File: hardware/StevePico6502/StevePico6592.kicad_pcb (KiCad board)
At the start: 2 copper layers, 145.3 x 124 mm, 41 parts, among them J1 GPIOB, J10 FTDI Power, J2 GPIOA, J3 Conn_02x16_Odd_Even, J4 ROM SELECT, J5 RAM SELECT, J6 Expansion, J7 IO SELECT, J8 CLK SELECT, J9 FTDI Connector, SW1 SW_Push, U1 W65C02S, U2 28C256, U3 CY62256-70PC, U4 W65C22S, U5 74HC00, U6 W6551, X1 CXO_DIP14, Y1 1.843

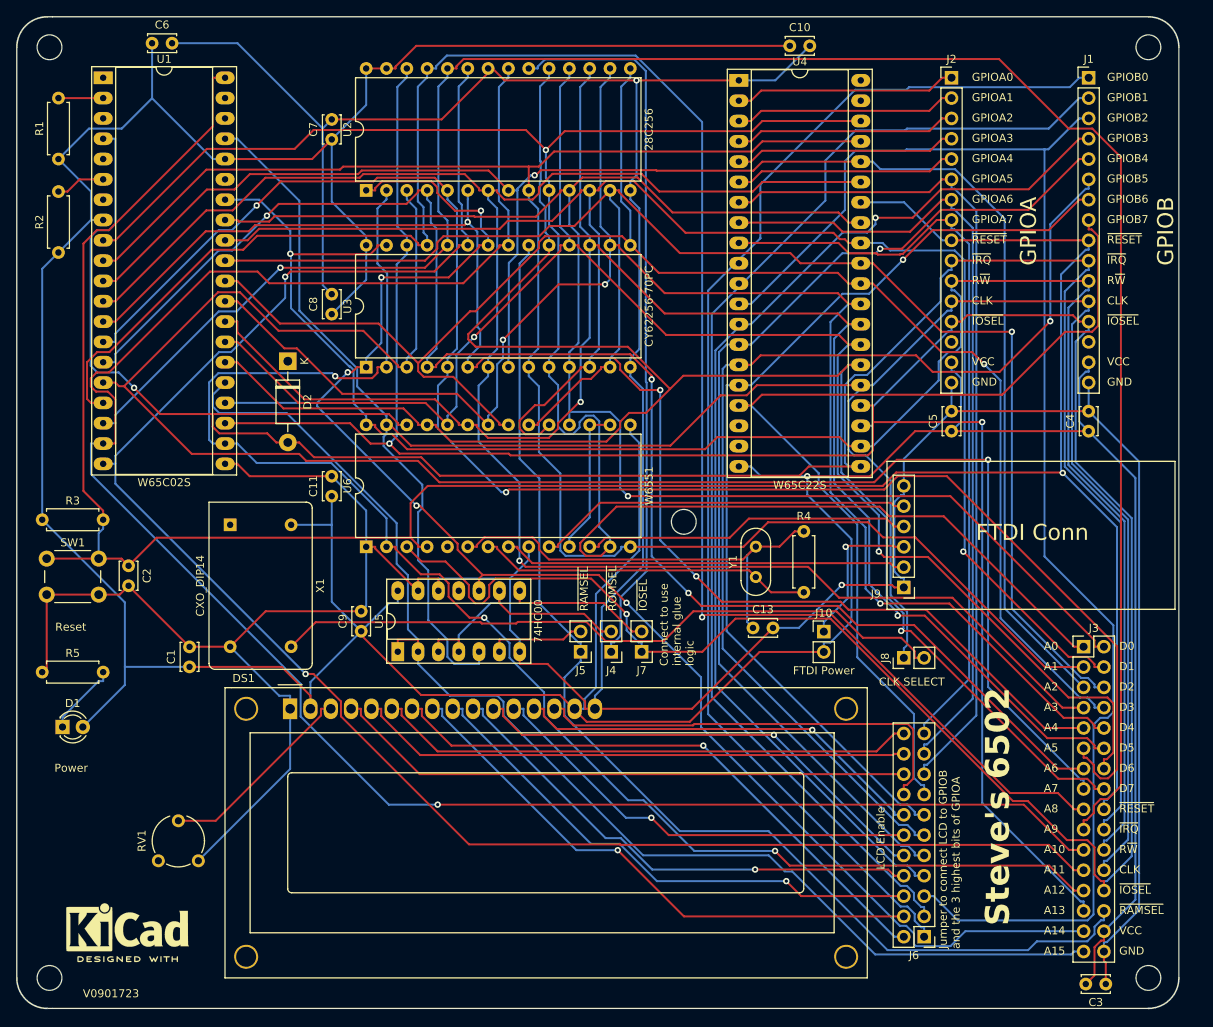
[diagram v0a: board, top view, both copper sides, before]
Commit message: 'V091723'
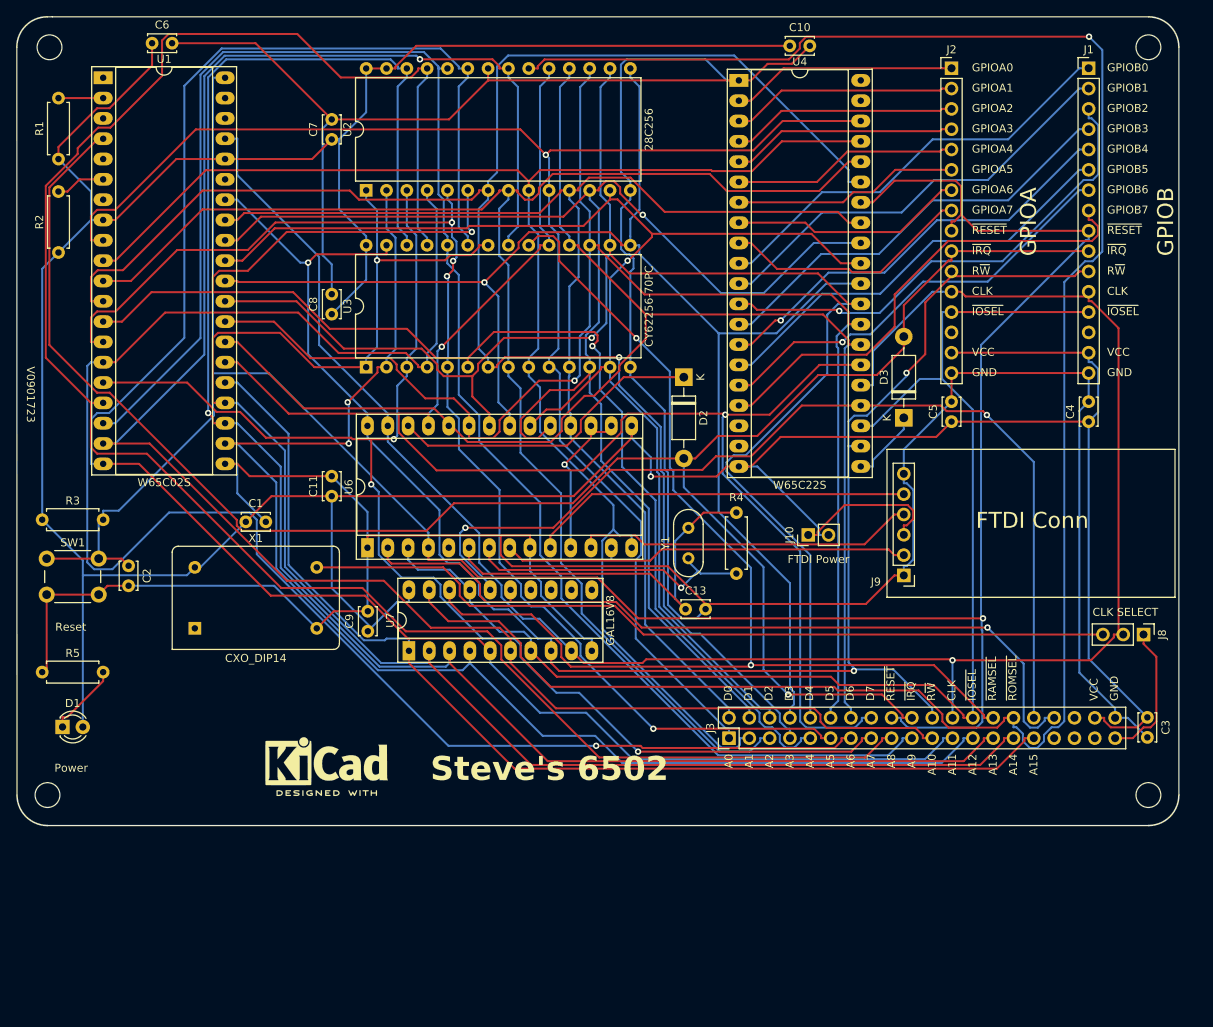
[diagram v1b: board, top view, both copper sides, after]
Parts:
- removed DS1: WC1602A, Display:WC1602A
- removed J4: ROM SELECT, Connector_PinHeader_2.54mm:PinHeader_1x02_P2.54mm_Vertical
- removed J5: RAM SELECT, Connector_PinHeader_2.54mm:PinHeader_1x02_P2.54mm_Vertical
- removed J6: Expansion, Connector_PinHeader_2.54mm:PinHeader_2x11_P2.54mm_Vertical
- removed J7: IO SELECT, Connector_PinHeader_2.54mm:PinHeader_1x02_P2.54mm_Vertical
- removed RV1: 10k, Potentiometer_THT:Potentiometer_Piher_PT-6-V_Vertical
- removed U5: 74HC00, Package_DIP:DIP-14_W7.62mm_Socket_LongPads
- added D3: SB140, Diode_THT:D_DO-41_SOD81_P10.16mm_Horizontal, F.Cu at (159.8, 83.2)
- added U7: GAL16V8, Package_DIP:DIP-20_W7.62mm_Socket_LongPads, F.Cu at (97.9, 112.3)
- J3: value Conn_02x16_Odd_Even -> Conn_02x20_Odd_Even; footprint Connector_PinHeader_2.54mm:PinHeader_2x16_P2.54mm_Vertical -> Connector_PinHeader_2.54mm:PinHeader_2x20_P2.54mm_Vertical
- J8: footprint Connector_PinHeader_2.54mm:PinHeader_1x02_P2.54mm_Vertical -> Connector_PinHeader_2.54mm:PinHeader_1x03_P2.54mm_Vertical
- U6: footprint Package_DIP:DIP-28_W15.24mm -> Package_DIP:DIP-28_W15.24mm_Socket_LongPads
- moved D2 49.5 mm to (132.3, 78.1)
- moved J3 45.8 mm to (137.9, 123.2), turned to 90 degrees
- moved C3 34.2 mm to (190.2, 120.6), turned to -90 degrees
- moved REF** 32.4 mm to (87.6, 126.1)
- moved J8 30.1 mm to (189.7, 110.2), turned to -90 degrees
- moved C1 19.4 mm to (77.5, 96.2), turned to 0 degrees
- moved X1 13.7 mm to (71.2, 109.5), turned to 0 degrees
- moved J10 12.2 mm to (147.8, 97.8), turned to 90 degrees
- moved C13 8.75 mm to (132.5, 107.1)
- moved R4 8.75 mm to (138.8, 102.6)
- moved Y1 8.75 mm to (132.8, 100.7)
- moved J9 1.50 mm to (159.8, 102.8)
- moved C4 1.19 mm to (182.9, 83.6)
- moved C5 1.19 mm to (165.7, 83.6)
- moved J1 1.19 mm to (182.9, 39.5)
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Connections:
- J3 pad 30: VCC -> /~{ROMSEL}
- J3 pad 32: GND -> /6522SEL
- J8 pad 1: /CLK -> /CLK_ALT
- J8 pad 2: /CLK_INT -> /CLK
- U4 pad 21: /~{IRQ} -> Net-(D3-K)
- U4 pad 24: /A13 -> /6522SEL
- U6 pad 2: /A12 -> /ACIASEL
- U6 pad 26: /~{IRQ} -> Net-(D2-K)
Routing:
- net /~{ROMSEL}: track 90.5 -> 255.3 mm, vias 0 -> 1
- net /6522SEL: track 0.00 -> 121.9 mm, vias 0 -> 2
- net /GPIOB2: track 180.4 -> 61.5 mm, vias 0 -> 1
- net /GPIOB0: track 155.6 -> 53.8 mm
- net /ACIASEL: track 0.00 -> 100.8 mm, vias 0 -> 1
- net /GPIOB1: track 148.6 -> 53.8 mm
- net VCC: track 564.8 -> 481.1 mm
- net /GPIOB3: track 136.5 -> 53.8 mm, vias 1 -> 0
- net /GPIOB5: track 135.1 -> 53.8 mm, vias 1 -> 0
- net /GPIOA5: track 106.5 -> 28.3 mm
- net /GPIOB4: track 130.9 -> 53.8 mm
- net /LCD_D0: track 73.8 -> 0.00 mm, vias 1 -> 0
- net /LCD_RS: track 73.0 -> 0.00 mm
- net /GPIOA6: track 102.0 -> 29.2 mm
- net /LCD_D1: track 70.2 -> 0.00 mm, vias 1 -> 0
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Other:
- board size 145.3 x 124 mm -> 145.3 x 101.1 mm
- board text removed: "Connect to use internal glue logic"
- board text removed: "Jumper to connect LCD to GPIOB and the 3 highest bits of GPIOA"
- board text removed: "LCD Enable"
